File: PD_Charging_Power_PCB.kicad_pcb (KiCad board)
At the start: 2 copper layers, 28 x 30 mm, 34 parts, among them J1 105450-0101, Q1 CJQ4459, Q2 2N7002KDW, U1 STUSB4500

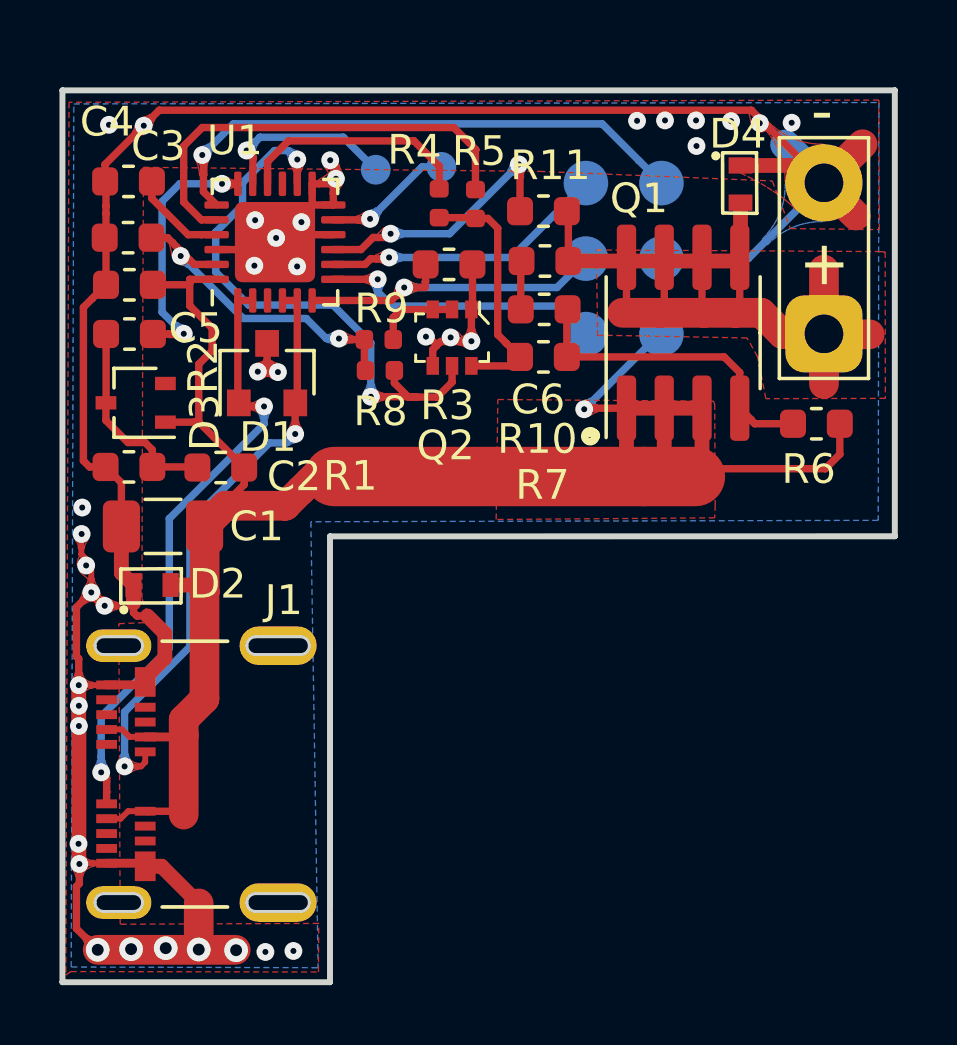
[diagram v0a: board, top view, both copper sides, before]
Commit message: Ruan: modify for V0.1
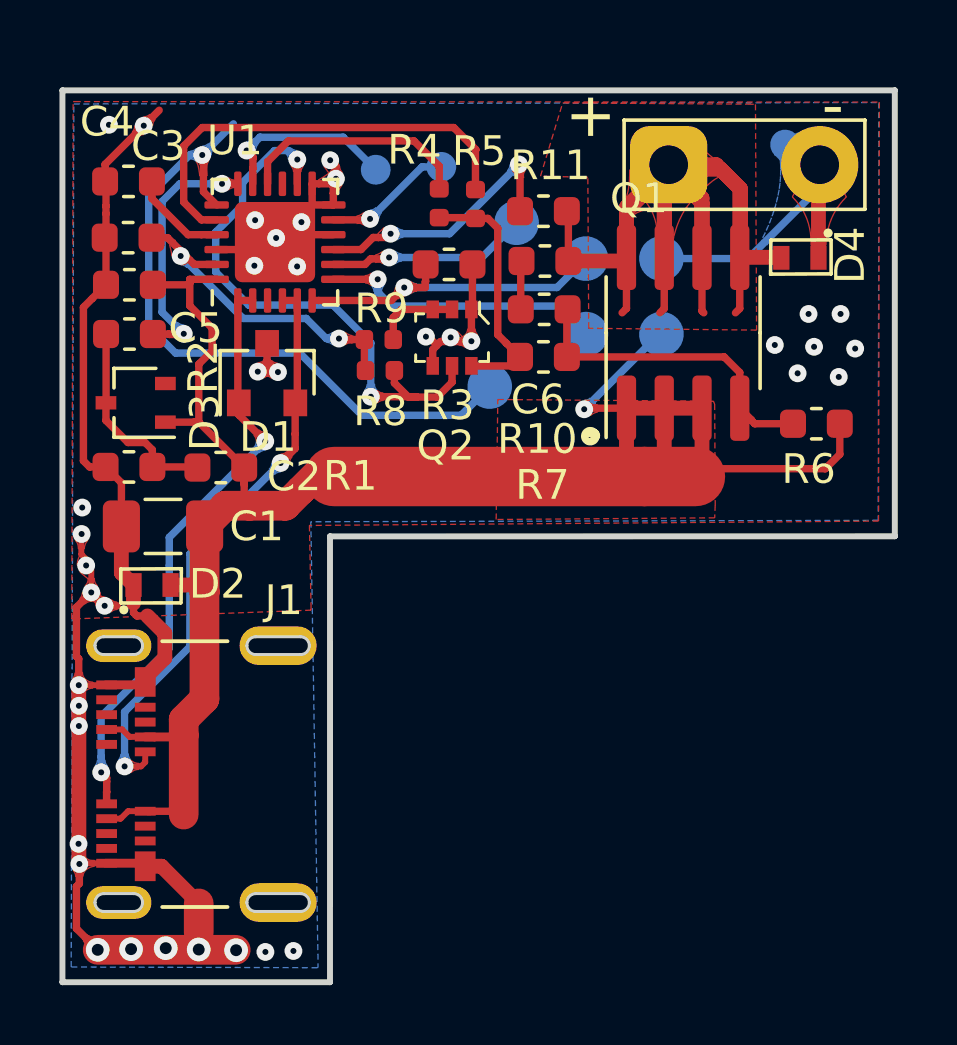
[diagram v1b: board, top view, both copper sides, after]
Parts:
- moved INT1 8.96 mm to (121.8, 146.8)
- moved TP8 7.72 mm to (127.8, 139.4), turned to 0 degrees
- moved SDA1 2.69 mm to (122.7, 141.3)
- moved D4 2.31 mm to (131.6, 142.5), turned to 0 degrees
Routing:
- net GND: track 107.8 -> 81.1 mm
- net Net-(C6-Pad1): track 31.1 -> 45.0 mm
- net Net-(INT1-Pad1): track 18.6 -> 23.2 mm
- net Net-(SDA1-Pad1): track 9.63 -> 6.75 mm

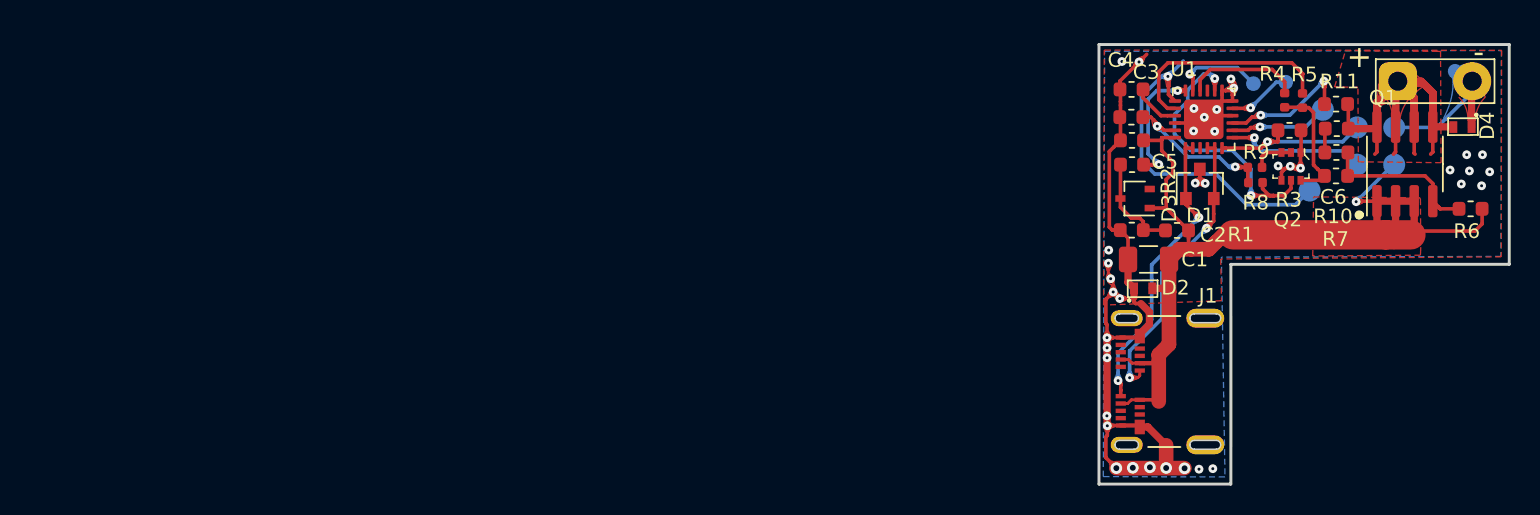
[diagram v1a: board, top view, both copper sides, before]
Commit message: Ruan: base ok V0.1
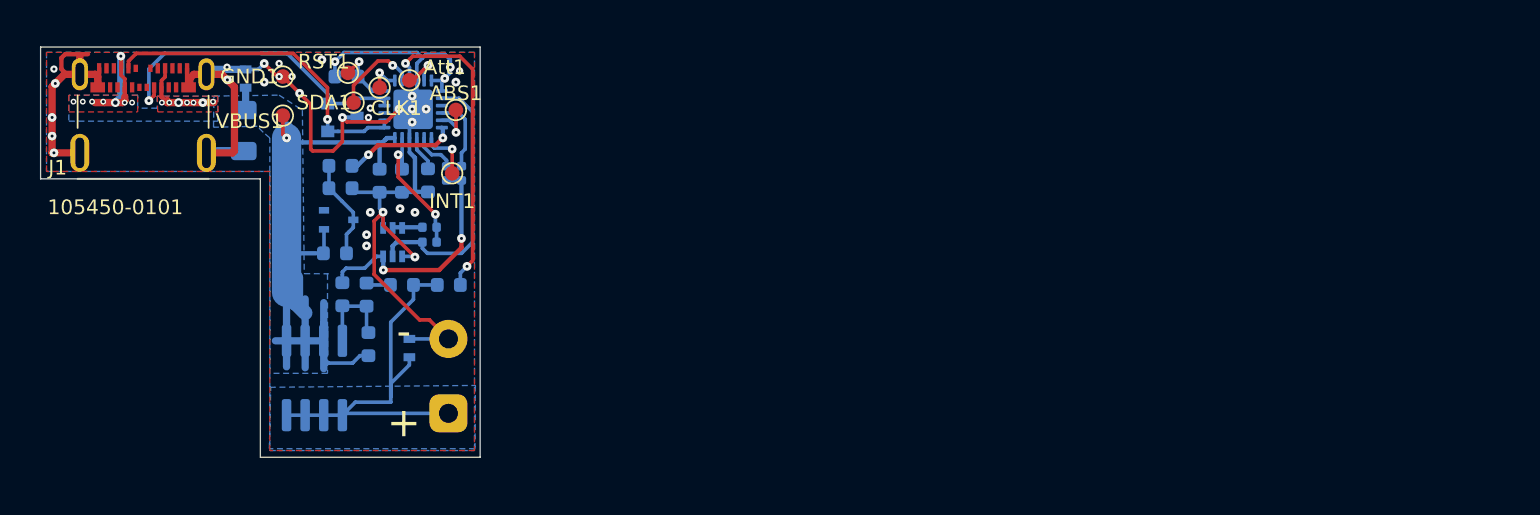
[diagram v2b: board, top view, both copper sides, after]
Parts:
- removed TP1: GND, TestPoint:TestPoint_Pad_D1.5mm
- added GND1: GND, TestPoint:TestPoint_Pad_D1.0mm, F.Cu at (51.7, 139.1)
- ABS1, Att1: moved to F.Cu
- C1, C2, C3, C4, C5, C6, D1, D2, D3, D4, Q1, R1, R10, R11, R2, R3, R4, R5, R6, R7, R8, R9, TP8, U1: moved to B.Cu
- CLK1, INT1, RST1, SDA1, VBUS1: footprint TestPoint:TestPoint_Pad_D1.5mm -> TestPoint:TestPoint_Pad_D1.0mm; moved to F.Cu
- J1: footprint RuanProject:MOLEX_105450-0101_modifyed -> RuanProject:MOLEX_105450-0101
- Q2: footprint digikey-footprints:SOT-363 -> RuanProject:SOT-363_SC-70-6; moved to B.Cu
- moved VBUS1 75.9 mm to (51.7, 141.7)
- moved Q1 75.8 mm to (53.8, 159.6), turned to 270 degrees
- moved R6 75.8 mm to (57.5, 157.3), turned to 90 degrees
- moved D4 73.0 mm to (60.3, 158.2), turned to 90 degrees
- moved J1 72.7 mm to (42.2, 142.3), turned to 0 degrees
- moved RST1 69.0 mm to (56.1, 138.8)
- moved TP8 68.6 mm to (63.0, 162.1), turned to 90 degrees
- moved R7 68.3 mm to (55.8, 153.9), turned to 90 degrees
- moved CLK1 66.9 mm to (58.3, 139.8)
- moved R10 66.9 mm to (57.4, 153.9), turned to 270 degrees
- moved SDA1 66.2 mm to (56.5, 140.8)
- moved C6 64.7 mm to (59.8, 153.3)
- moved R3 64.5 mm to (56.0, 139.1), turned to 180 degrees
- moved D2 63.4 mm to (49.1, 139.8), turned to 90 degrees
- moved C1 62.4 mm to (49.0, 142.8), turned to 90 degrees
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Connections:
- J1 pad S1: Net-(J1-PadS1) -> GND
- J1 pad S2: Net-(J1-PadS1) -> GND
- J1 pad S3: Net-(J1-PadS1) -> GND
- J1 pad S4: Net-(J1-PadS1) -> GND
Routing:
- net GND: track 81.1 -> 105.7 mm, vias 38 -> 34
- net Net-(INT1-Pad1): track 23.2 -> 3.66 mm
- net Net-(C6-Pad1): track 45.0 -> 28.3 mm
- net Net-(R11-Pad2): track 9.08 -> 21.5 mm
- net Net-(R5-Pad2): track 15.0 -> 2.92 mm
- net Net-(Q2-Pad6): track 8.52 -> 16.5 mm, vias 0 -> 2
- net Net-(CLK1-Pad1): track 9.51 -> 2.27 mm
- net Net-(R3-Pad1): track 11.3 -> 4.33 mm
- net Net-(Q1-Pad4): track 10.9 -> 6.09 mm
- net /CC2: track 19.7 -> 24.0 mm, vias 2 -> 1
- net Net-(ABS1-Pad1): track 6.19 -> 3.05 mm
- net Net-(R4-Pad2): track 7.92 -> 5.07 mm
- net /CC1: track 20.3 -> 22.7 mm, vias 2 -> 1
- net Net-(Att1-Pad1): track 4.37 -> 2.83 mm
- net VBUS: track 72.7 -> 73.8 mm, vias 1 -> 16
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- added copper zone on B.Cu, net Net-(C6-Pad1)
- added copper zone on B.Cu, net VBUS
- removed copper zone on F.Cu, net Net-(C6-Pad1)
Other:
- board size 28 x 30 mm -> 30 x 28 mm
